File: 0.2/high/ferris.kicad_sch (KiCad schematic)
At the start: 102 parts, among them J1 TYPE-C-31-M-12, K0_0 KEYSW, K0_1 KEYSW, K0_2 KEYSW, K0_3 KEYSW, K0_4 KEYSW, K0_5 KEYSW, K0_6 KEYSW, K0_7 KEYSW, K0_8 KEYSW, K0_9 KEYSW, K1_0 KEYSW, K1_1 KEYSW, K1_2 KEYSW, K1_3 KEYSW, K1_4 KEYSW, K1_5 KEYSW, K1_6 KEYSW, K1_7 KEYSW, K1_8 KEYSW, K1_9 KEYSW, K2_0 KEYSW, K2_1 KEYSW, K2_2 KEYSW, K2_3 KEYSW, K2_4 KEYSW, K2_5 KEYSW, K2_6 KEYSW, K2_7 KEYSW, K2_8 KEYSW, K2_9 KEYSW, K3_3 KEYSW, K3_4 KEYSW, K3_5 KEYSW, K3_6 KEYSW, Q1 PDTC123JT,215, SW1 B3U-1000P, U1 STM32F072CBT6, U2 MCP23017-E/SO, U3 MCP1700T-3302E/TT, U4 SRV05-4

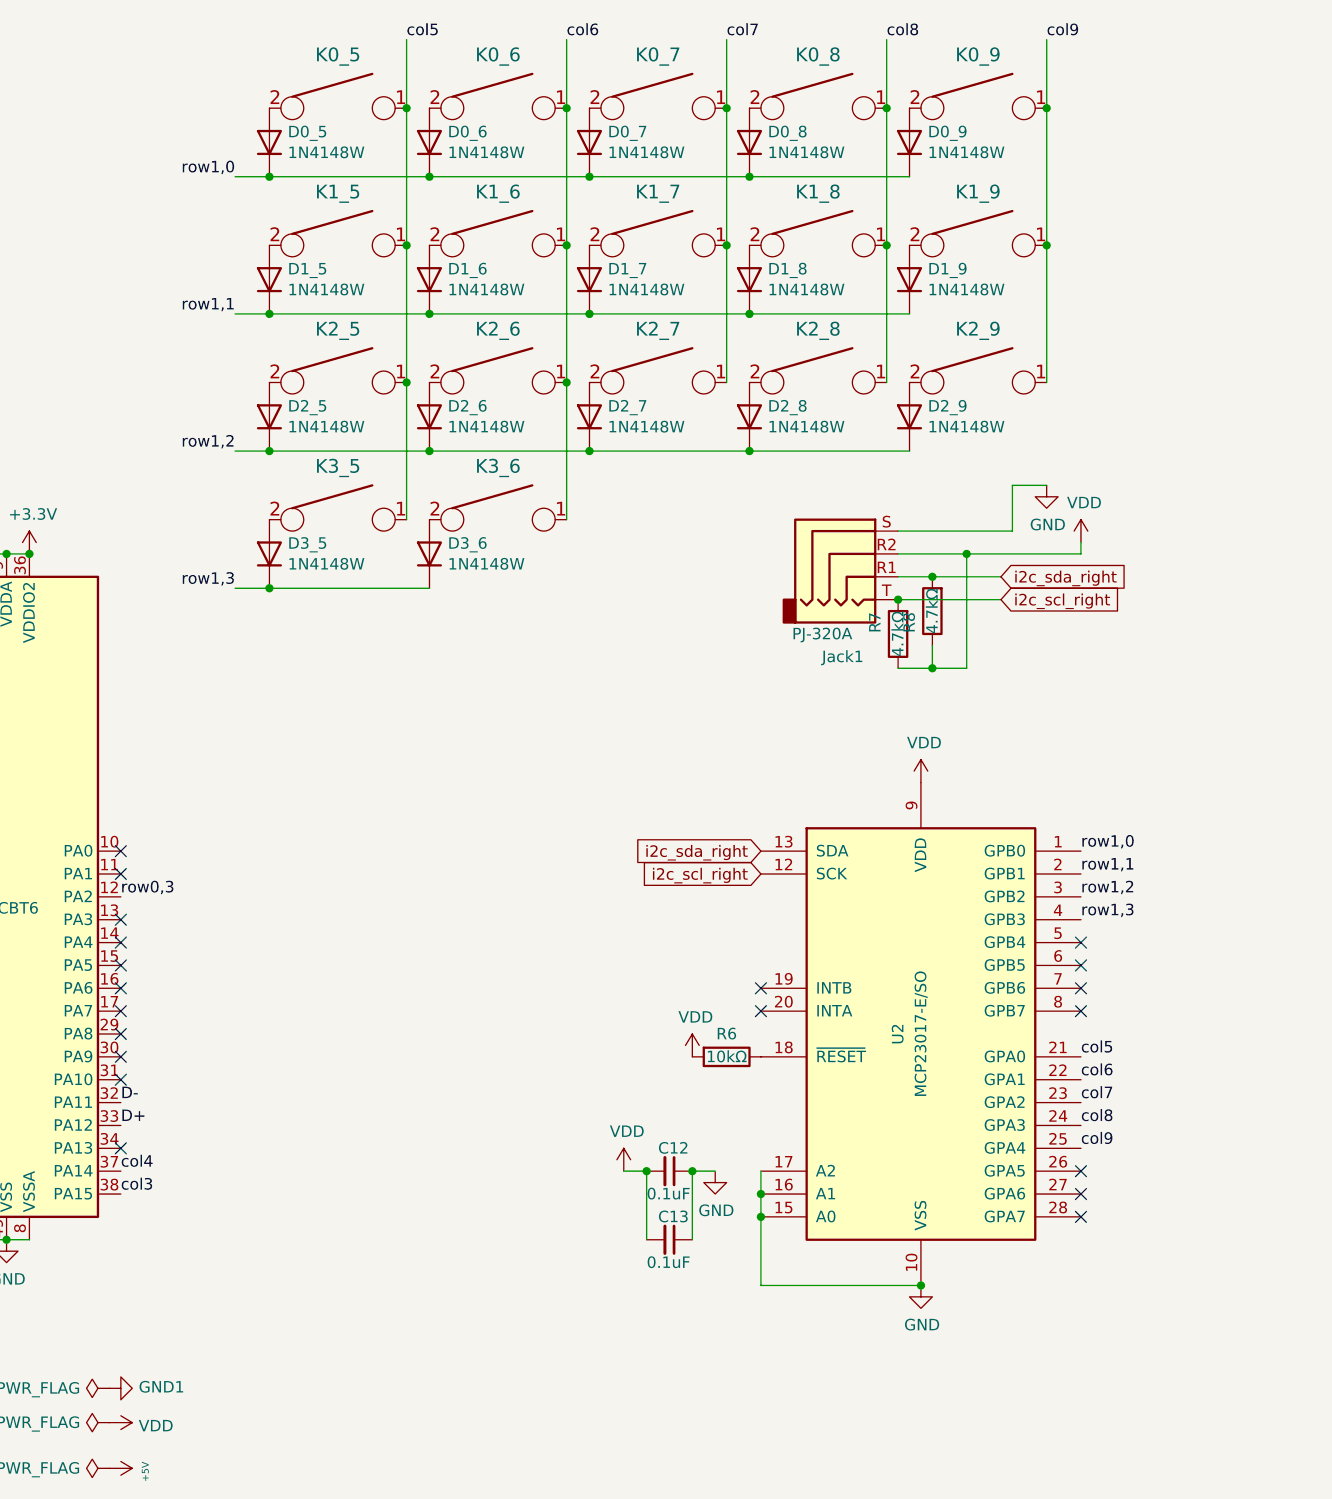
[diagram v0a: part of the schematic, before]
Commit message: Again, initiate reversible
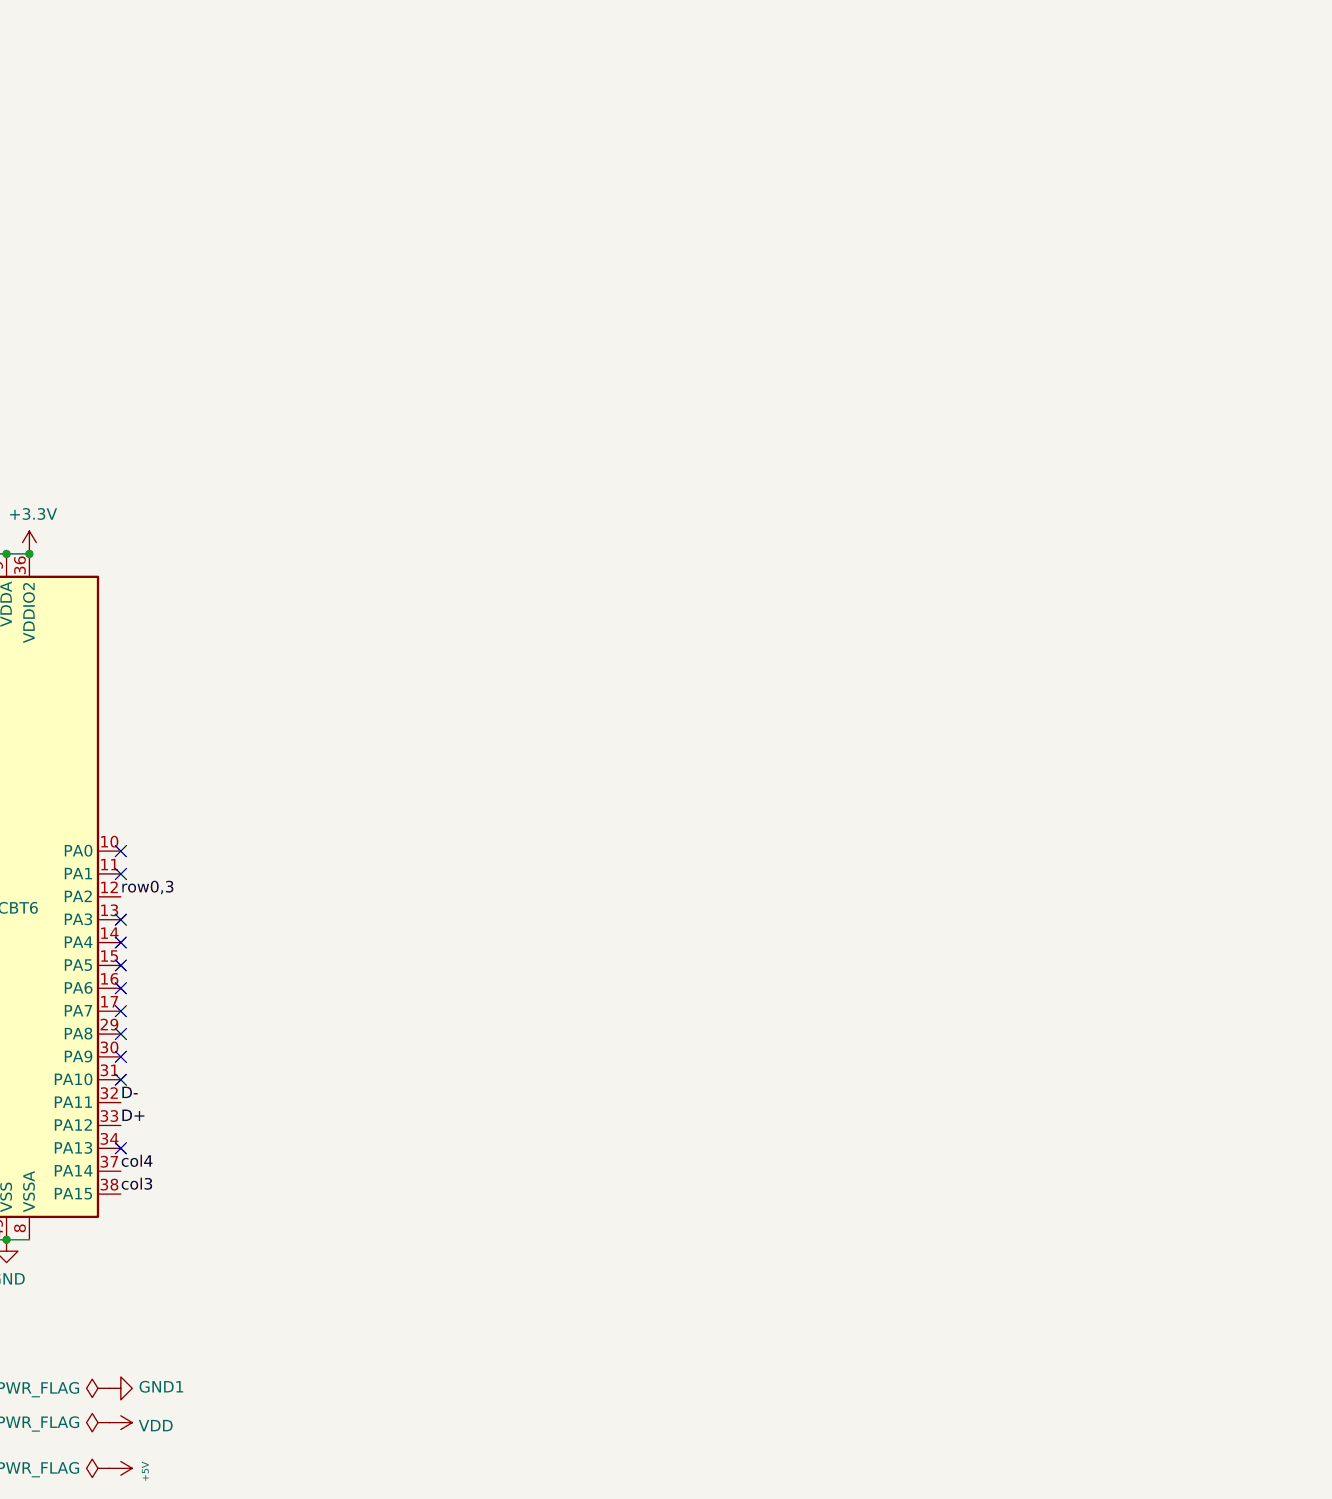
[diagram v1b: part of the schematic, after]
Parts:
- removed C12, C13: 0.1uF, Capacitor_SMD:C_0805_2012Metric_Pad1.15x1.40mm_HandSolder, symbol Device:C_Small
- removed D0_5, D0_6, D0_7, D0_8, D0_9, D1_5, D1_6, D1_7, D1_8, D1_9, D2_5, D2_6, D2_7, D2_8, D2_9, D3_5, D3_6: 1N4148W, Diode_SMD:D_SOD-123, symbol Device:D
- removed Jack1: PJ-320A, kbd:TRRS-PJ-320A, symbol Connector:AudioJack4
- removed K0_5, K0_6, K0_7, K0_8, K0_9, K1_5, K1_6, K1_7, K1_8, K1_9, K2_5, K2_6, K2_7, K2_8, K2_9, K3_5, K3_6: KEYSW, switches:MX, symbol keyboard_parts:KEYSW
- removed R6: 10kΩ, Resistor_SMD:R_0805_2012Metric_Pad1.15x1.40mm_HandSolder, symbol Device:R
- removed R7, R8: 4.7kΩ, Resistor_SMD:R_0805_2012Metric_Pad1.15x1.40mm_HandSolder, symbol Device:R
- removed U2: MCP23017-E/SO, Package_SO:SOIC-28W_7.5x17.9mm_P1.27mm, symbol Interface_Expansion:MCP23017_SO
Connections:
- no-connect marks 37 -> 28
